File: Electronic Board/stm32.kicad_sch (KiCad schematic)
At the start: 15 parts, among them U6 STM32F446ZCTx

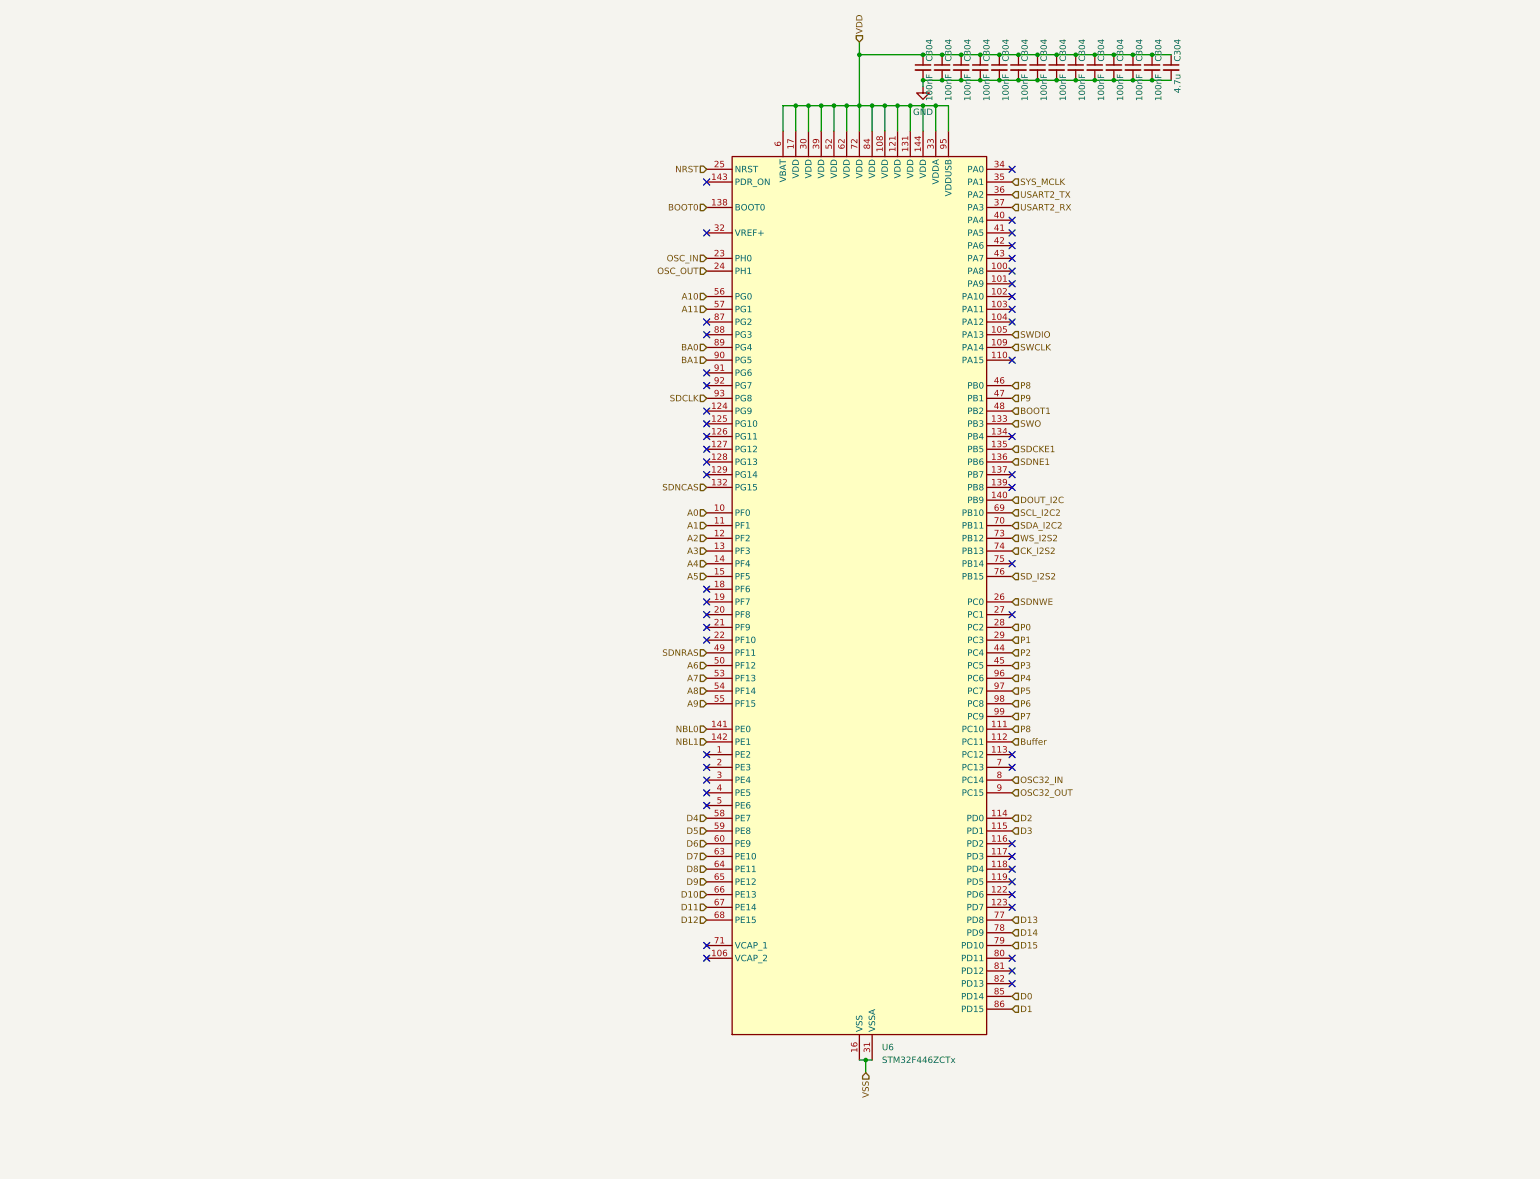
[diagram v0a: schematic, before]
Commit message: Add files via upload
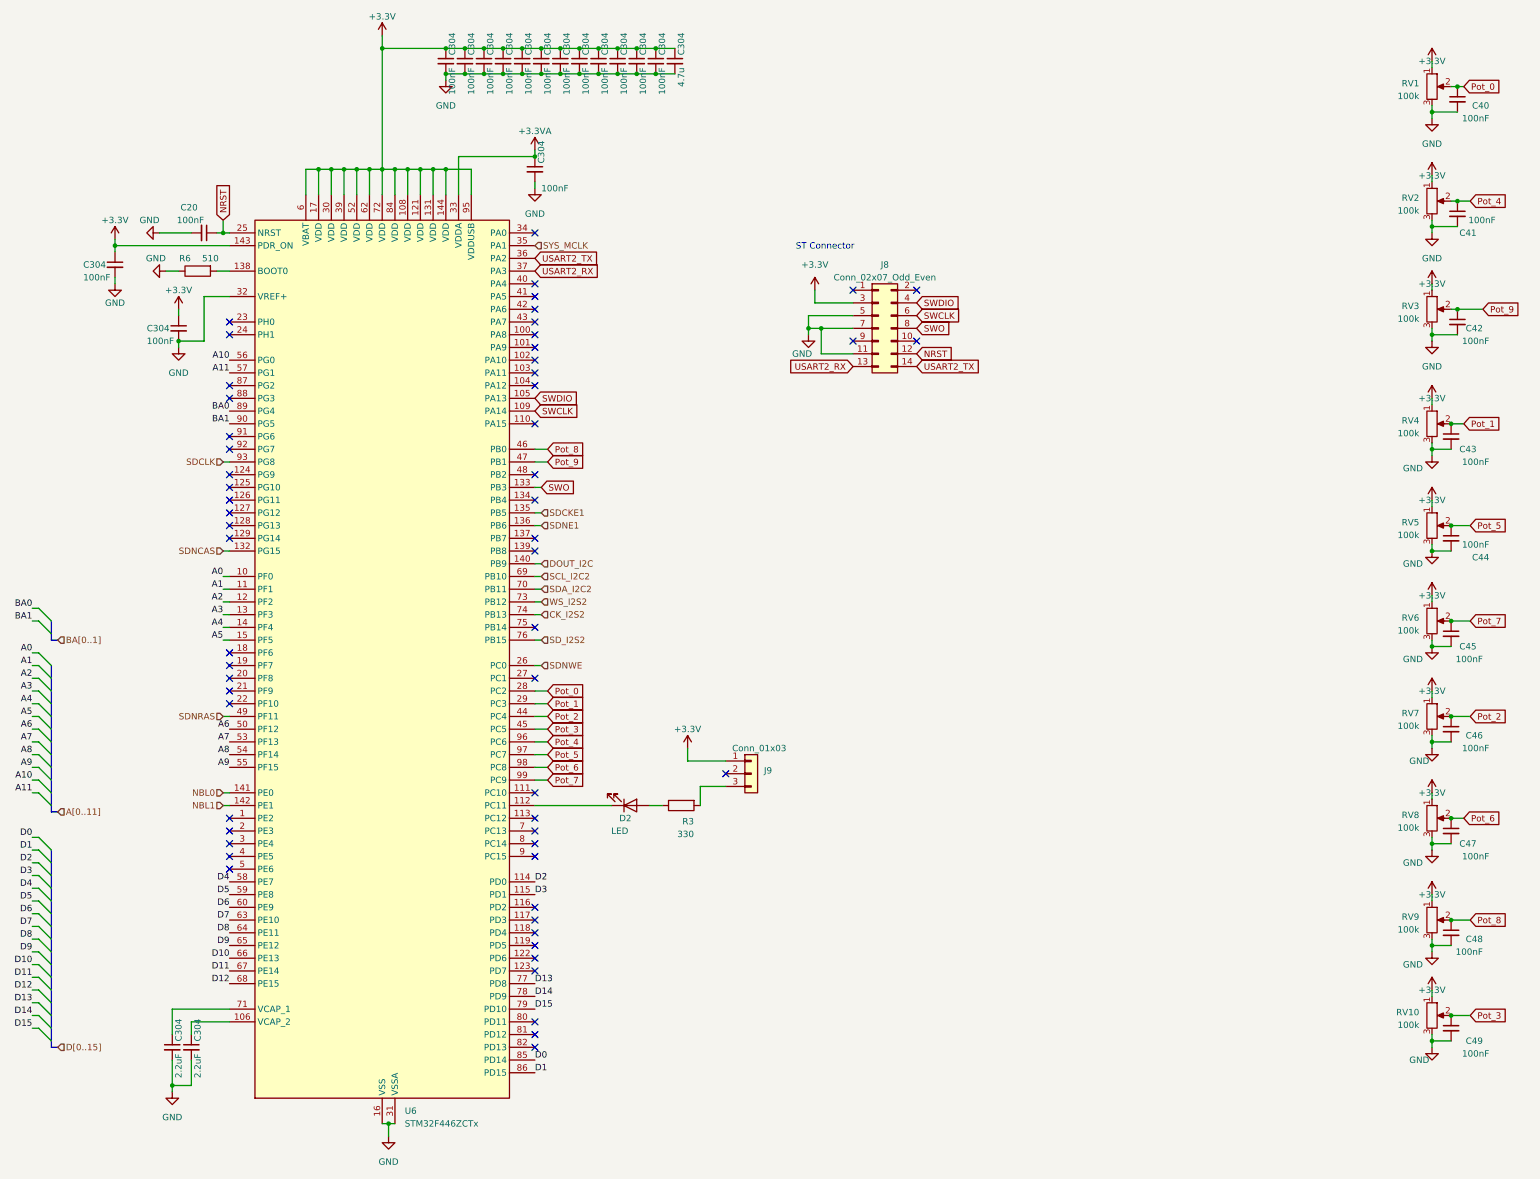
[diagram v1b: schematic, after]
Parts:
- added C20, C304 (x2), C40, C41, C42, C43, C44, C45, C46, C47, C48, C49: 100nF, Capacitor_SMD:C_0402_1005Metric_Pad0.74x0.62mm_HandSolder, symbol Device:C_Small
- added C304 (x2): 2.2uF, Capacitor_SMD:C_0402_1005Metric_Pad0.74x0.62mm_HandSolder, symbol Device:C_Small
- added D2: LED, LED_SMD:LED_0402_1005Metric_Pad0.77x0.64mm_HandSolder, symbol Device:LED
- added J8: Conn_02x07_Odd_Even, Connector_PinHeader_1.27mm:PinHeader_2x07_P1.27mm_Vertical_SMD, symbol Connector_Generic:Conn_02x07_Odd_Even
- added J9: Conn_01x03, Connector_JST:JST_XH_S3B-XH-A-1_1x03_P2.50mm_Horizontal, symbol Connector_Generic:Conn_01x03
- added R3: 330, Resistor_SMD:R_0201_0603Metric_Pad0.64x0.40mm_HandSolder, symbol Device:R
- added R6: 510, Resistor_SMD:R_0201_0603Metric_Pad0.64x0.40mm_HandSolder, symbol Device:R
- added RV1, RV10, RV2, RV3, RV4, RV5, RV6, RV7, RV8, RV9: 100k, Library:Potentiometer_Alpha_RD901F-40-00D_Single_Vertical, symbol Device:R_Potentiometer
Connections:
- net VSS is gone; now on net GND: U6.107 (VSS), U6.120 (VSS), U6.130 (VSS), U6.16 (VSS), U6.31 (VSSA), U6.38 (VSS), U6.51 (VSS), U6.61 (VSS), U6.83 (VSS), U6.94 (VSS)
- net GND: now also U6.32 (VREF+), C20.2, C304.2, C304.2, C304.2, C304.2, C40.2, C41.2, C42.2, C43.2, C44.2, C45.2, C46.2, C47.2, C48.2, C49.2, J8.11 (Pin_11), J8.5 (Pin_5), J8.7 (Pin_7), R6.1, RV1.3, RV10.3, RV2.3, RV3.3, RV4.3, RV5.3, RV6.3, RV7.3, RV8.3, RV9.3
- net NRST: now also C20.1, J8.12 (Pin_12)
- net SWCLK: now also J8.6 (Pin_6)
- net SWDIO: now also J8.4 (Pin_4)
- net SWO: now also J8.8 (Pin_8)
- net USART2_RX: now also J8.13 (Pin_13)
- net USART2_TX: now also J8.14 (Pin_14)
- net at U6.106 (VCAP_2): now also C304.1
- net +3.3V: now reaches U6.143 (PDR_ON)
- net +3.3V: now also C304.1, C304.1, C304.1, C304.1, C304.1, C304.1, C304.1, C304.1, C304.1, C304.1, C304.1, C304.1, C304.1, U6.108 (VDD), U6.121 (VDD), U6.131 (VDD), U6.144 (VDD), U6.17 (VDD), U6.30 (VDD), U6.39 (VDD), U6.52 (VDD), U6.6 (VBAT), U6.62 (VDD), U6.72 (VDD), U6.84 (VDD), U6.95 (VDDUSB), C304.1, C304.1, J8.3 (Pin_3), J9.1 (Pin_1), RV1.1, RV10.1, RV2.1, RV3.1, RV4.1, RV5.1, RV6.1, RV7.1, RV8.1, RV9.1
- net at U6.71 (VCAP_1): now also C304.1
- net BOOT0: no longer names the net of U6.138 (BOOT0)
- net BOOT0: now also R6.2
- net BOOT1: no longer names the net of U6.48 (PB2)
- net Buffer: no longer names the net of U6.112 (PC11)
- net Buffer: now also D2.1 (K)
- net OSC32_IN: no longer names the net of U6.8 (PC14)
- net OSC32_OUT: no longer names the net of U6.9 (PC15)
- net OSC_IN: no longer names the net of U6.23 (PH0)
- net OSC_OUT: no longer names the net of U6.24 (PH1)
- net P0 renamed Pot_0
- net Pot_0: now also C40.1, RV1.2
- net P1 renamed Pot_1
- net Pot_1: now also C43.1, RV4.2
- net P2 renamed Pot_2
- net Pot_2: now also C46.1, RV7.2
- net P3 renamed Pot_3
- net Pot_3: now also C49.1, RV10.2
- net P4 renamed Pot_4
- net Pot_4: now also C41.1, RV2.2
- net P5 renamed Pot_5
- net Pot_5: now also C44.1, RV5.2
- net P6 renamed Pot_6
- net Pot_6: now also C47.1, RV8.2
- net P7 renamed Pot_7
- net Pot_7: now also C45.1, RV6.2
- net P8: no longer names the net of U6.111 (PC10)
- net P8: no longer U6.46 (PB0)
- net P9 renamed Pot_9
- net Pot_9: now also C42.1, RV3.2
- removed net VDD: C304.1, C304.1, C304.1, C304.1, C304.1, C304.1, C304.1, C304.1, C304.1, C304.1, C304.1, C304.1, C304.1, C304.1, U6.108 (VDD), U6.121 (VDD), U6.131 (VDD), U6.144 (VDD), U6.17 (VDD), U6.30 (VDD), U6.33 (VDDA), U6.39 (VDD), U6.52 (VDD), U6.6 (VBAT), U6.62 (VDD), U6.72 (VDD), U6.84 (VDD), U6.95 (VDDUSB)
- new net: D2.2 (A), R3.1
- new net: J9.3 (Pin_3), R3.2
- new net +3.3VA: C304.1, U6.33 (VDDA)
- new net Pot_8: C48.1, RV9.2, U6.46 (PB0)
- no-connect marks 51 -> 58
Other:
- note added: "ST Connector"
- moved on the sheet: C304, U6
